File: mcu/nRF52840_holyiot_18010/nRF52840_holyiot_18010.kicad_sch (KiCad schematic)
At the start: 3 parts

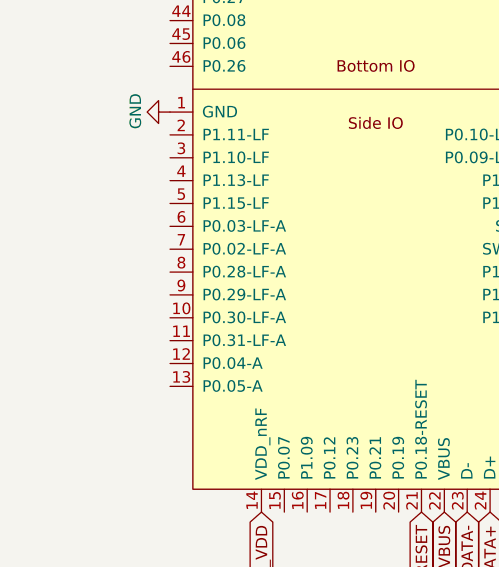
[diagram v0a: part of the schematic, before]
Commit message: update battery module
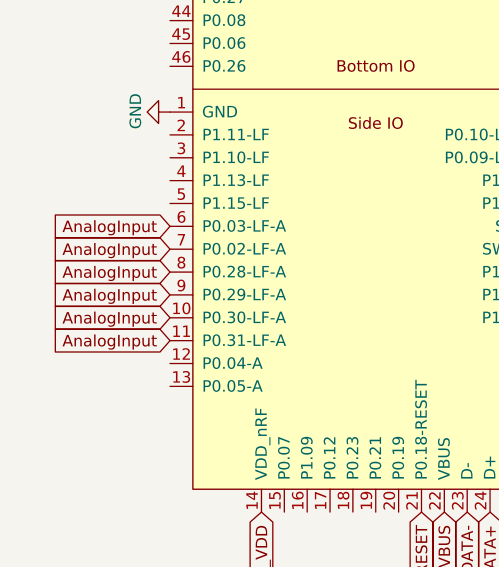
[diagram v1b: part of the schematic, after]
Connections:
- net AnalogInput: now reaches MCU_U1.10 (P0.30-LF-A)
- net AnalogInput: now also MCU_U1.11 (P0.31-LF-A), MCU_U1.6 (P0.03-LF-A), MCU_U1.7 (P0.02-LF-A), MCU_U1.8 (P0.28-LF-A), MCU_U1.9 (P0.29-LF-A)
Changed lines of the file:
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@@
+		)
+	)
+	(global_label "AnalogInput"
+		(shape input)
+		(at 68.58 82.55 180)
+		(fields_autoplaced yes)
+		(effects
+			(font
+				(size 1.27 1.27)
+			)
+			(justify right)
+		)
+		(property "Intersheetrefs" "${INTERSHEET_REFS}"
+			(at 54.4675 82.55 0)
+			(effects
+				(font
+					(size 1.27 1.27)
+				)
+				(justify right)
+				(hide yes)
+			)
+		)
+	)
+	(global_label "AnalogInput"
+		(shape input)
+		(at 68.58 92.71 180)
+		(fields_autoplaced yes)
+		(effects
+			(font
+				(size 1.27 1.27)
+			)
+			(justify right)
+		)
+		(property "Intersheetrefs" "${INTERSHEET_REFS}"
+			(at 54.4675 92.71 0)
+			(effects
+				(font
+					(size 1.27 1.27)
+				)
+				(justify right)
+				(hide yes)
+			)
 		)
 	)
@@
 		)
 	)
+	(global_label "AnalogInput"
+		(shape input)
+		(at 68.58 90.17 180)
+		(fields_autoplaced yes)
+		(effects
+			(font
+				(size 1.27 1.27)
+			)
+			(justify right)
+		)
+		(property "Intersheetrefs" "${INTERSHEET_REFS}"
+			(at 54.4675 90.17 0)
+			(effects
+				(font
+					(size 1.27 1.27)
+				)
+				(justify right)
+				(hide yes)
+			)
+		)
+	)
+	(global_label "AnalogInput"
+		(shape input)
+		(at 68.58 80.01 180)
+		(fields_autoplaced yes)
+		(effects
+			(font
+				(size 1.27 1.27)
+			)
+			(justify right)
+		)
+		(property "Intersheetrefs" "${INTERSHEET_REFS}"
+			(at 54.4675 80.01 0)
+			(effects
+				(font
+					(size 1.27 1.27)
+				)
+				(justify right)
+				(hide yes)
+			)
+		)
+	)
 	(global_label "SWC"
 		(shape input)
@@
 				(hide yes)
 			)
+		)
+	)
+	(global_label "AnalogInput"
+		(shape input)
+		(at 68.58 85.09 180)
+		(fields_autoplaced yes)
+		(effects
+			(font
+				(size 1.27 1.27)
+			)
+			(justify right)
+		)
+		(property "Intersheetrefs" "${INTERSHEET_REFS}"
+			(at 54.4675 85.09 0)
+			(effects
+				(font
+					(size 1.27 1.27)
+				)
+				(justify right)
+				(hide yes)
+			)
+		)
+	)
+	(global_label "AnalogInput"
+		(shape input)
+		(at 68.58 87.63 180)
+		(fields_autoplaced yes)
+		(effects
+			(font
+				(size 1.27 1.27)
+			)
+			(justify right)
+		)
+		(property "Intersheetrefs" "${INTERSHEET_REFS}"
+			(at 54.4675 87.63 0)
+			(effects
+				(font
+					(size 1.27 1.27)
+				)
+				(justify right)
+				(hide yes)
+			)
